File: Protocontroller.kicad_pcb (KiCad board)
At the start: 2 copper layers, 50.1 x 27.3 mm, 34 parts, among them J2 Conn_01x14_Socket, J3 Conn_01x14_Socket, J4 Conn_01x04, J7 Conn_02x08_Odd_Even, U1 AP2112K-3.3TRG1, U4 SN74AHCT08PWR, U5 SN74AHCT245PWR, U6 74AHCT374

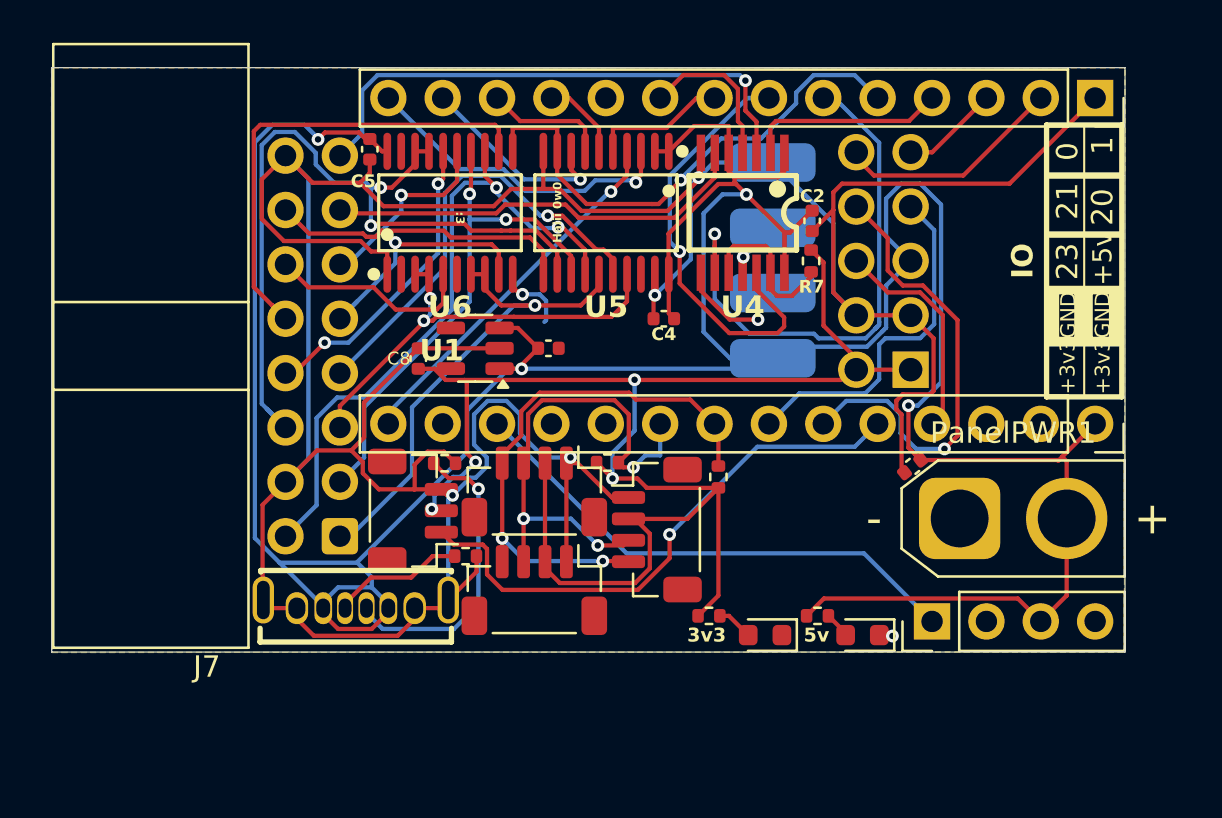
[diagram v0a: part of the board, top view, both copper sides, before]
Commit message: fix files
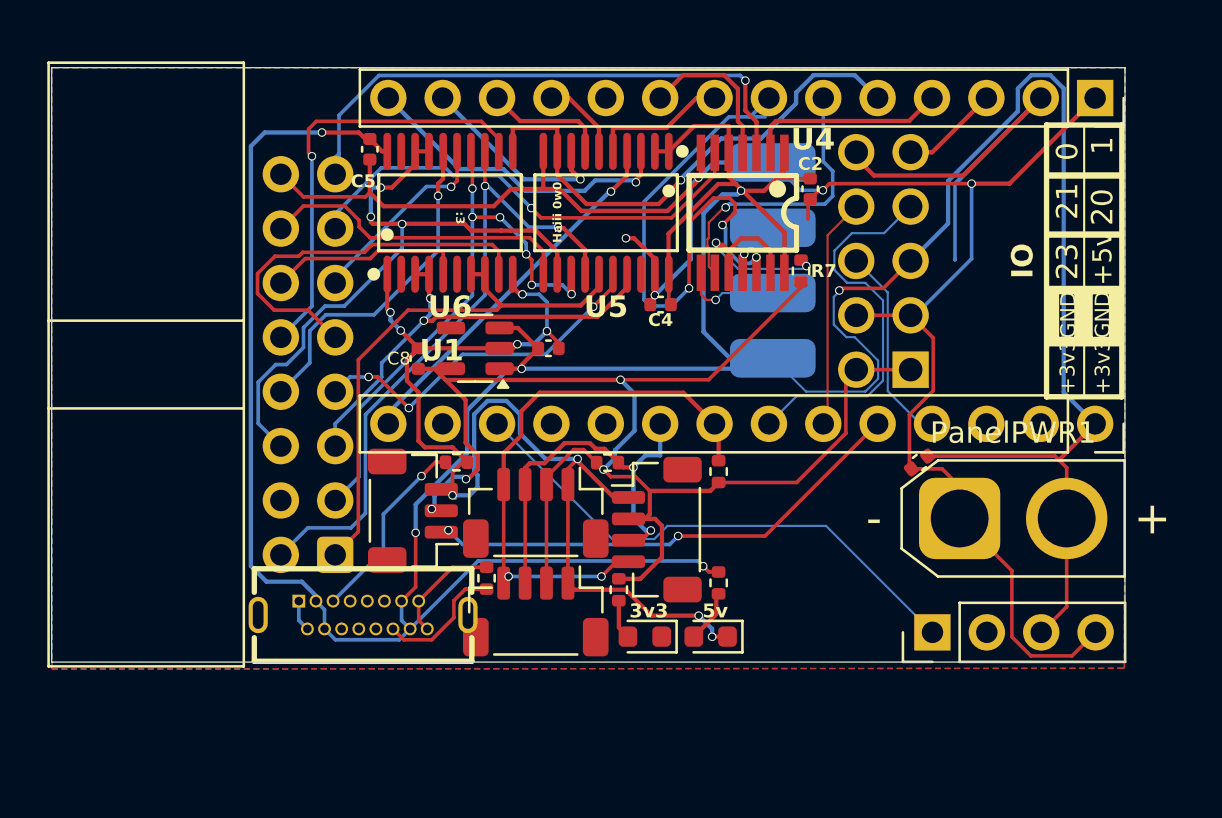
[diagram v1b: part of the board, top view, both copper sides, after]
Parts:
- removed PWRINPUT1: USB-C-TH_TYPE-C-6PLCH10.0-073, Protocontroller:USB-C-TH_TYPE-C-6P-LC6.8-073
- added J1: USB_C_Receptacle_USB2.0_16P, Protocontroller:USB-TH_TYPE-C-16PFS-LCH7.45-IPX8, F.Cu at (124.5, 47.5)
- C2, C4, C5: value 0.1uF_0402 -> 100nF_0402
- PanelPWR1: value XT30U-M -> XT30U-M.G.B
- moved D2 7.09 mm to (140.7, 48.5)
- moved D1 5.62 mm to (137.7, 48.5)
- moved R11 4.87 mm to (141.1, 46.0), turned to -90 degrees
- moved R8 4.38 mm to (136.4, 46.3), turned to -90 degrees
- moved Qr 2.54 mm to (113.6, 46.1)
- moved C2 1.50 mm to (145.4, 27.6)
- moved R1 1.42 mm to (130.3, 45.8), turned to -90 degrees
- moved I2C-2 1.00 mm to (132.6, 47.3)
- moved I2C-3 1.00 mm to (132.6, 42.7)
- moved J7 0.90 mm to (123.2, 44.7)
- moved C4 0.68 mm to (138.4, 33.0)
- moved R7 0.66 mm to (145.0, 31.4)
- moved R4 0.55 mm to (128.9, 40.4)
- moved FanHeader1 0.51 mm to (151.1, 48.3)
- moved C3 0.37 mm to (150.5, 40.4)
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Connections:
- I2C-1 pad MP: (no net) -> unconnected-(I2C-1-PadMP)_1
- I2C-2 pad MP: (no net) -> GND
- I2C-3 pad MP: (no net) -> unconnected-(I2C-3-PadMP)
- R7 pad 1: Net-(U4-3B) -> +3.3V
- R7 pad 2: +3.3V -> Net-(U4-3B)
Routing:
- net GND: track 179.4 -> 154.6 mm, vias 6 -> 14
- net +5V: track 168.0 -> 180.8 mm, vias 4 -> 6
- net /FLEXIO_SCK: track 25.5 -> 13.6 mm
- net /Digital1: track 21.6 -> 10.8 mm, vias 1 -> 0
- net /RX: track 11.5 -> 20.7 mm
- net /PANEL_G2: track 38.3 -> 30.2 mm, vias 2 -> 3
- net /PANEL_ADX0: track 11.9 -> 18.4 mm, vias 1 -> 0
- net Net-(J1-CC1): track 14.2 -> 8.94 mm
- net /FLEXIO_MOSI: track 21.4 -> 26.5 mm, vias 1 -> 3
- net /SDA: track 24.0 -> 19.0 mm, vias 3 -> 2
- net /PANEL_B2: track 21.7 -> 16.8 mm, vias 1 -> 3
- net +3.3V: track 73.9 -> 70.4 mm
- net /Mic1: track 26.1 -> 23.0 mm, vias 1 -> 2
- net Net-(U4-3B): track 7.59 -> 10.5 mm, vias 0 -> 2
- net /PANEL_ADX1: track 23.0 -> 20.4 mm, vias 0 -> 1
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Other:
- board size 50.1 x 27.3 mm -> 50.1 x 27.8 mm
